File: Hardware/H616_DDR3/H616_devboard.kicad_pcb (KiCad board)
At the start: 8 copper layers, 50 x 50 mm, 169 parts, among them J1 Micro_SD_Card_Det2, J2 HDMI_D_1.4, J3 USB_C_Receptacle_USB2.0, J4 USB_C_Receptacle_USB2.0, J5 Conn_01x40_Pin, Q1 AO3420_C358680, Q2 AO3401A, Q3 AO3401A, SW1 CK_KMS2xxG, U1 H616, U10 D3V3XA4B10LP, U11 D3V3XA4B10LP, U2 K4B8G1646D, U3 AXP305, U4 SW6206, U6 KLMBG2JETD-B041, U7 AP6256, U8 D3V3XA4B10LP, U9 D3V3XA4B10LP, Y1 24MHz

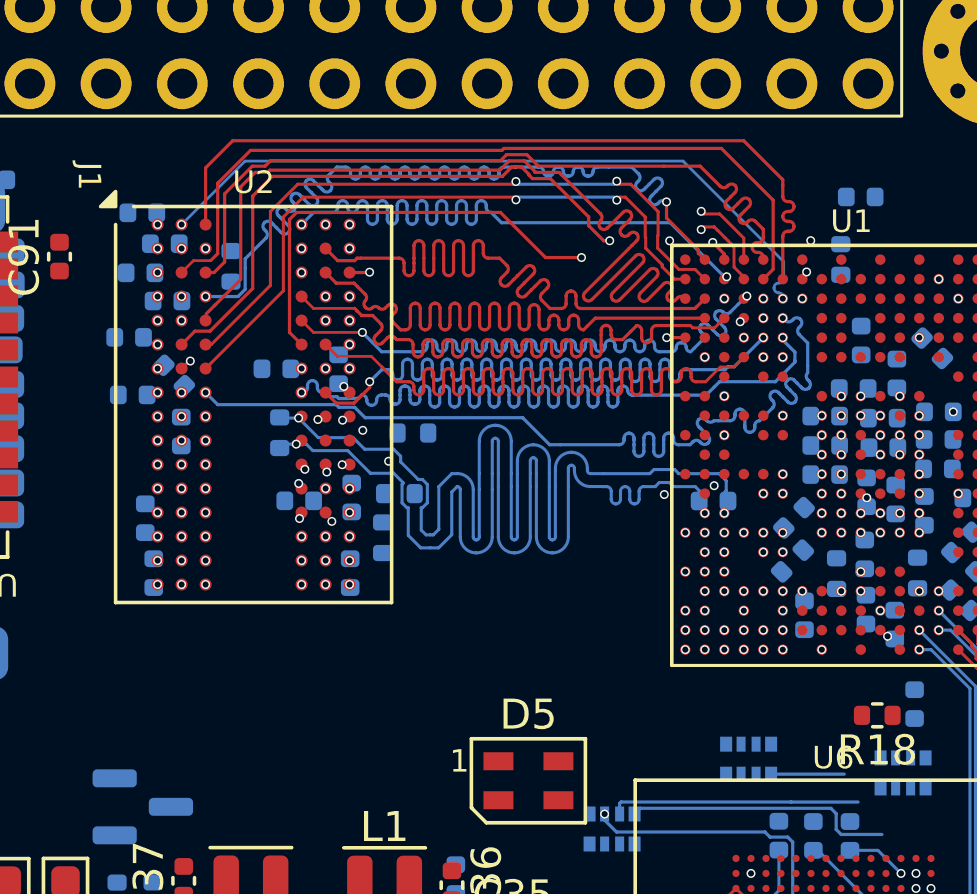
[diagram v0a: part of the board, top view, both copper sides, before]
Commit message: ddr trace
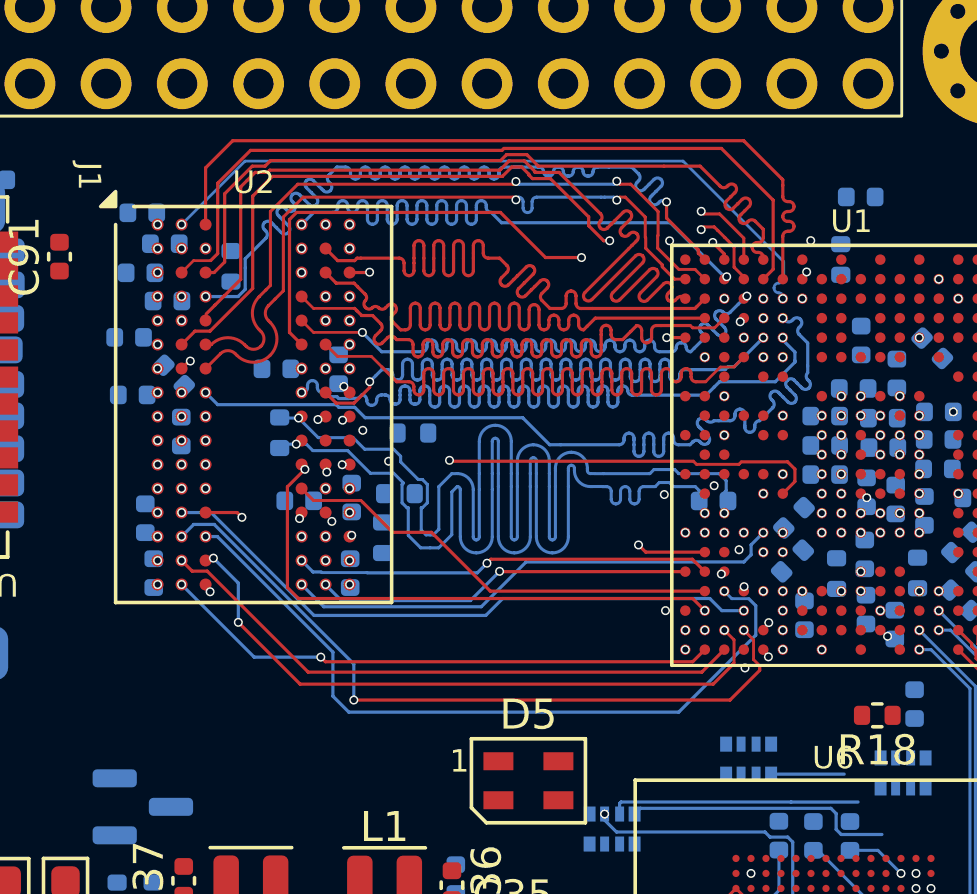
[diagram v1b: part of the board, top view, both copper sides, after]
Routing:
- net /DRAM/SA2: track 0.00 -> 24.9 mm
- net /DRAM/SA5: track 0.00 -> 24.5 mm, vias 2 -> 3
- net /DRAM/SA9: track 0.00 -> 21.4 mm, vias 2 -> 3
- net /DRAM/SA0: track 0.00 -> 21.2 mm
- net /DRAM/SA3: track 0.00 -> 20.6 mm
- net /DRAM/SA7: track 0.00 -> 19.9 mm, vias 2 -> 1
- net /DRAM/SA1: track 0.00 -> 19.6 mm
- net /DRAM/SA12: track 0.00 -> 19.5 mm
- net /DRAM/SRST: track 0.00 -> 18.7 mm
- net /DRAM/SA13: track 0.00 -> 18.5 mm
- net /DRAM/SA10: track 0.00 -> 18.4 mm
- net /DRAM/SA6: track 0.00 -> 18.2 mm
- net /DRAM/SA14: track 0.00 -> 16.9 mm
- net /DRAM/SA15: track 0.00 -> 14.9 mm, vias 2 -> 0
- net /DRAM/SA11: track 0.00 -> 14.0 mm
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
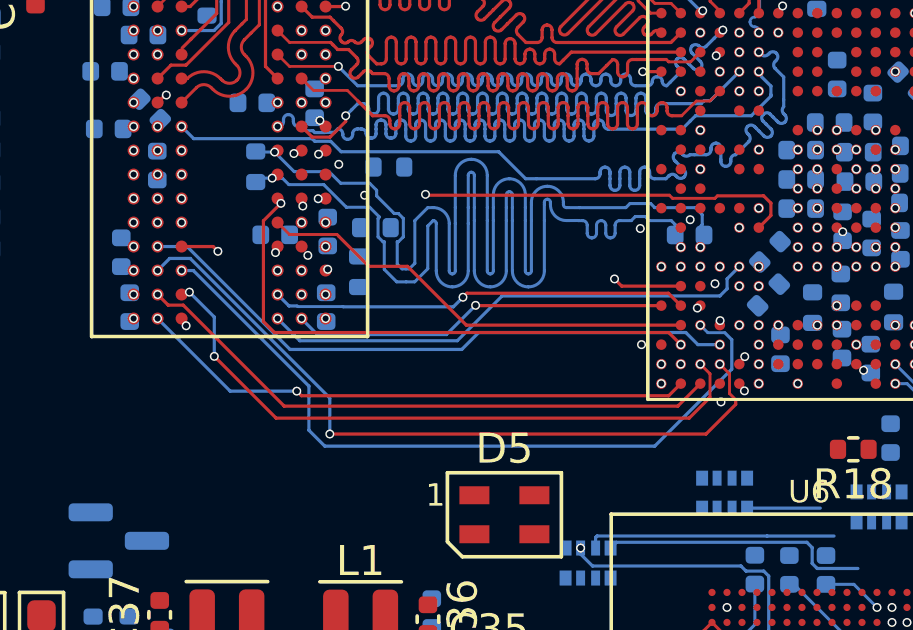
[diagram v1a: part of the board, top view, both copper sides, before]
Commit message: ddr trace
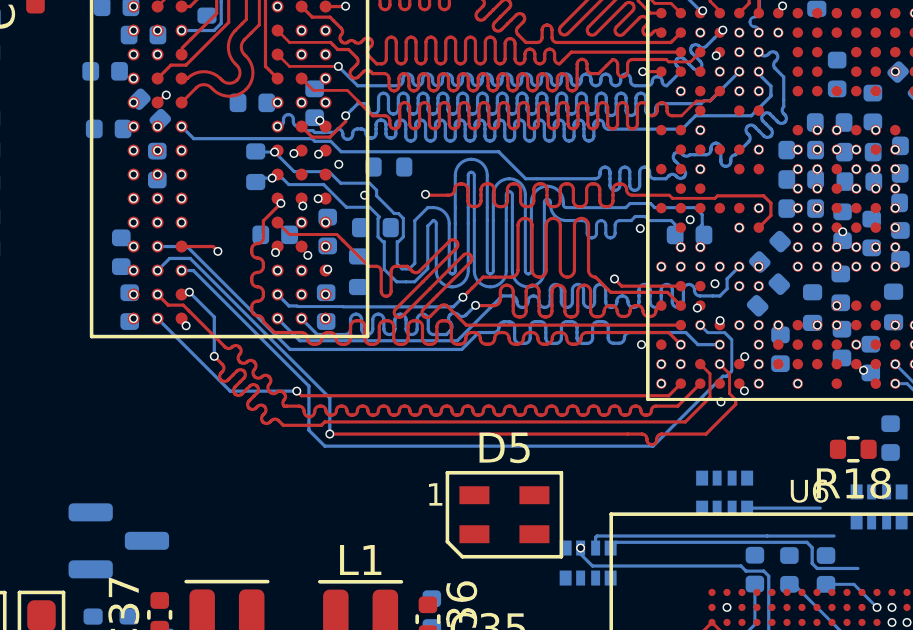
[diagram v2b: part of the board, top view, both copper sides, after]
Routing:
- net /DRAM/SA15: track 14.9 -> 27.2 mm
- net /DRAM/SA8: track 12.6 -> 24.6 mm
- net /DRAM/SA11: track 14.0 -> 24.8 mm
- net /DRAM/SA4: track 13.0 -> 21.6 mm
- net /DRAM/SA10: track 18.4 -> 26.9 mm
- net /DRAM/SA14: track 16.9 -> 24.7 mm
- net /DRAM/SA6: track 18.2 -> 25.6 mm
- net /DRAM/SA7: track 19.9 -> 26.8 mm
- net /DRAM/SA3: track 20.6 -> 24.8 mm
- net /DRAM/SA9: track 21.4 -> 24.9 mm, vias 3 -> 2
- net /DRAM/SA12: track 19.5 -> 22.7 mm
- net /DRAM/SA13: track 18.5 -> 21.4 mm
- net /DRAM/SA1: track 19.6 -> 21.5 mm
